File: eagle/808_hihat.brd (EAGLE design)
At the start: 100 x 80 mm, 103 parts, among them IC1 TL072P, IC3 TL071P, Q1 2N3904, Q10 2N3904, Q11 2N3904, Q12 2N3904, Q13 2N3906, Q14 2N3906, Q2 2N3904, Q3 2N3904, Q4 2N3904, Q5 2N3904, Q6 2N3904, Q7 2N3904, Q8 2N3904, Q9 2N3904

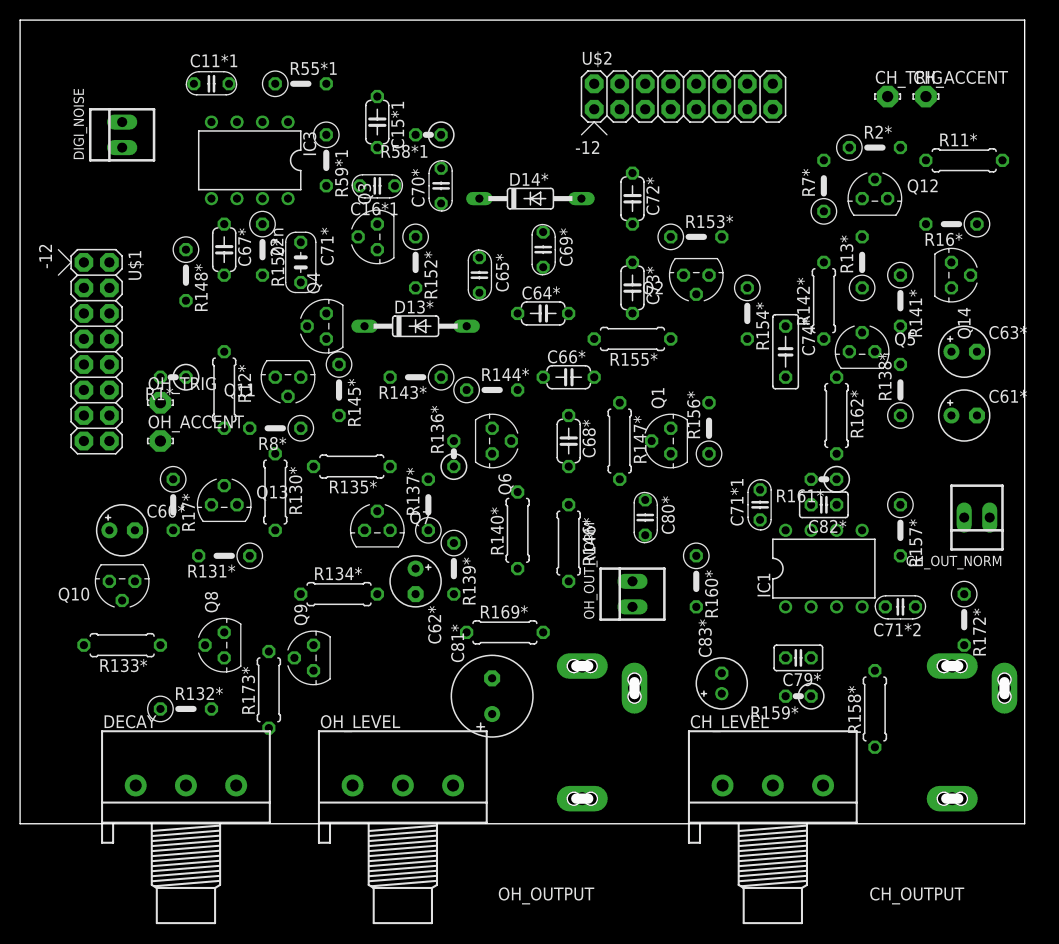
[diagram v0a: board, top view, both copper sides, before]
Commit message: 94pct6 ar
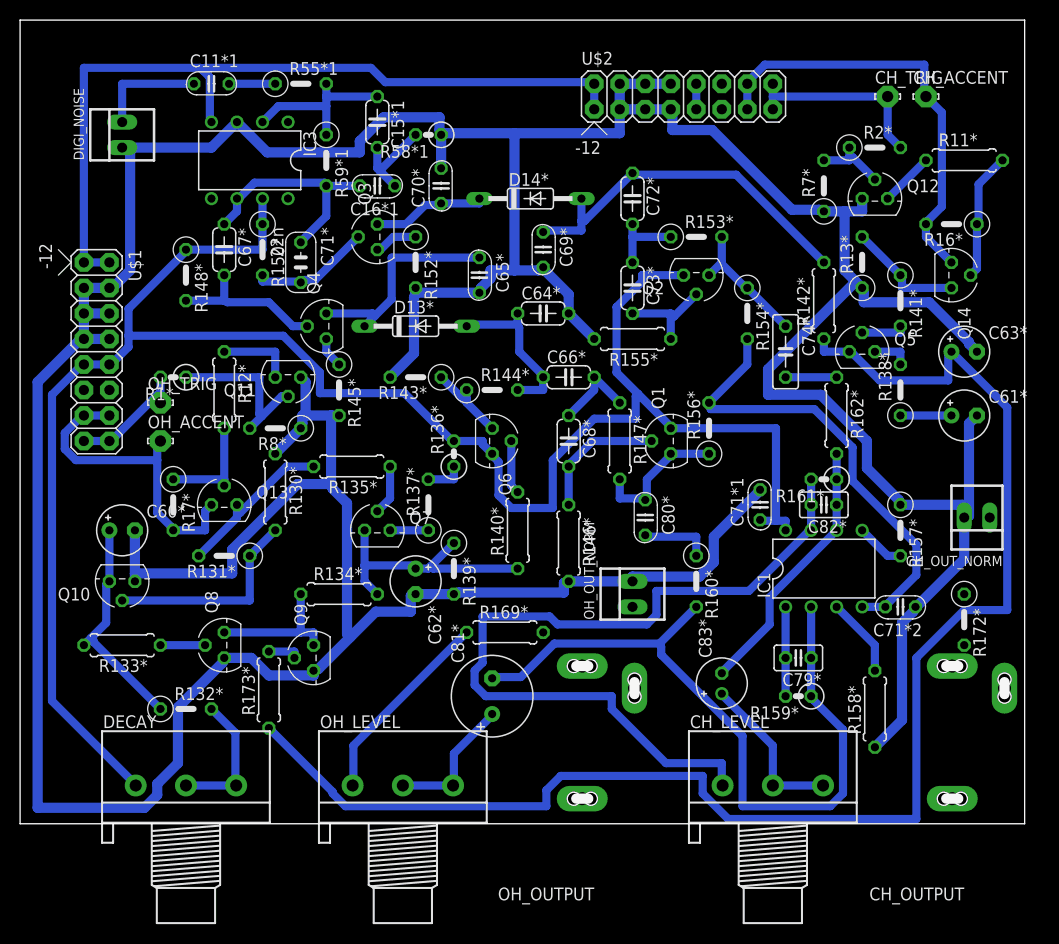
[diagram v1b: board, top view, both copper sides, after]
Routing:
- net GND: track 0.00 -> 484.9 mm
- net +12V: track 0.00 -> 195.1 mm
- net N$581: track 0.00 -> 145.7 mm
- net -12V: track 0.00 -> 128.0 mm
- net N$603: track 0.00 -> 81.5 mm
- net N$598: track 0.00 -> 73.3 mm
- net .: track 0.00 -> 43.1 mm
- net N$220: track 0.00 -> 36.9 mm
- net N$17: track 0.00 -> 32.0 mm
- net N$600: track 0.00 -> 28.9 mm
- net N$601: track 0.00 -> 26.6 mm
- net N$573: track 0.00 -> 25.8 mm
- net TO_HH: track 0.00 -> 22.8 mm
- net N$576: track 0.00 -> 22.4 mm
- net N$588: track 0.00 -> 21.6 mm
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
